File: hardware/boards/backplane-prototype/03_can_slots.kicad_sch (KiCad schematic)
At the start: 17 parts, among them J1 SLOT_1, J2 XY308-2.54-3P / EXTERNAL CAN, J3 SLOT_2, J4 SLOT_3, J6 SLOT_4, J7 SLOT_5, J8 SLOT_6, U5 TCAN3413DR

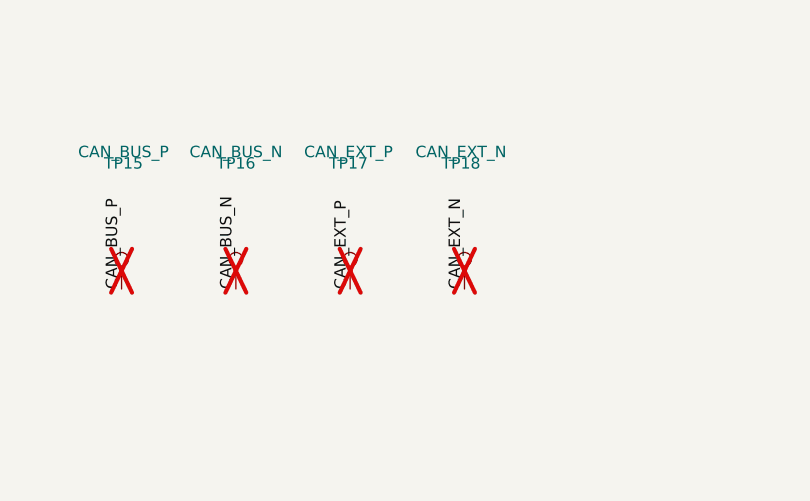
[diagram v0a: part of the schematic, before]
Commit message: checkpoint: save backplane layout updates
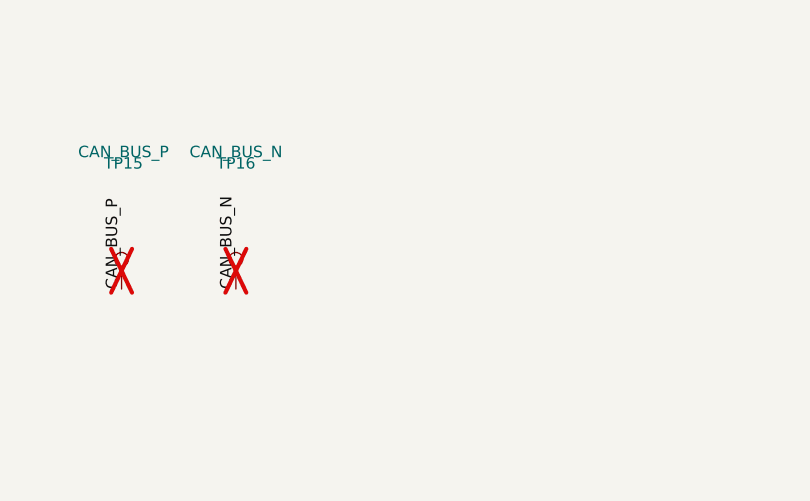
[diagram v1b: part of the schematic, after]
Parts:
- removed TP17: CAN_EXT_P, TestPoint:TestPoint_Pad_D1.5mm, symbol Connector:TestPoint
- removed TP18: CAN_EXT_N, TestPoint:TestPoint_Pad_D1.5mm, symbol Connector:TestPoint
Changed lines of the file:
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@@
-		)
-	)
-	(label "CAN_EXT_N"
-		(at 262.89 44.45 90)
-		(effects
-			(font
-				(size 1.27 1.27)
-			)
-			(justify left bottom)
 		)
 	)
@@
 	(label "CAN_BUS_P"
 		(at 39.37 132.08 0)
-		(effects
-			(font
-				(size 1.27 1.27)
-			)
-			(justify left bottom)
-		)
-	)
-	(label "CAN_EXT_P"
-		(at 250.19 44.45 90)
 		(effects
 			(font
@@
 	)
 	(symbol
-		(lib_id "Connector:TestPoint")
-		(at 262.89 44.45 0)
-		(unit 1)
-		(body_style 1)
-		(exclude_from_sim no)
-		(in_bom no)
-		(on_board yes)
-		(in_pos_files yes)
-		(dnp yes)
-		(property "Reference" "TP18"
-			(at 262.5 30.48 0)
-			(show_name no)
-			(do_not_autoplace no)
-			(effects
-				(font
-					(size 1.27 1.27)
-				)
-			)
-		)
-		(property "Value" "CAN_EXT_N"
-			(at 262.5 29.21 0)
-			(show_name no)
-			(do_not_autoplace no)
-			(effects
-				(font
-					(size 1.27 1.27)
-				)
-			)
-		)
-		(property "Footprint" "TestPoint:TestPoint_Pad_D1.5mm"
-			(at 267.58 45 0)
-			(hide yes)
-			(show_name no)
-			(do_not_autoplace no)
-			(effects
-				(font
-					(size 1.27 1.27)
-				)
-			)
-		)
-		(property "Datasheet" ""
-			(at 267.58 45 0)
-			(hide yes)
-			(show_name no)
-			(do_not_autoplace no)
-			(effects
-				(font
-					(size 1.27 1.27)
-				)
-			)
-		)
-		(property "Description" "test point"
-			(at 262.5 45 0)
-			(hide yes)
-			(show_name no)
-			(do_not_autoplace no)
-			(effects
-				(font
-					(size 1.27 1.27)
-				)
-			)
-		)
-		(pin "1"
-		)
-		(instances
-			(project "backplane-prototype"
-				(path "/348cc909-6345-4013-9bef-98714057a65b/eb7e4e77-e42b-4b43-976a-f7a3e8147b95"
-					(reference "TP18")
-					(unit 1)
-				)
-			)
-		)
-	)
-	(symbol
 		(lib_id "backplane-backpack:ACT1210D_1243")
 		(at 115.57 54.61 0)
@@
 					(unit 1)
 				)
-			)
-		)
-	)
-	(symbol
-		(lib_id "Connector:TestPoint")
-		(at 250.19 44.45 0)
-		(unit 1)
-		(body_style 1)
-		(exclude_from_sim no)
-		(in_bom no)
-		(on_board yes)
-		(in_pos_files yes)
-		(dnp yes)
-		(property "Reference" "TP17"
-			(at 250 30.48 0)
-			(show_name no)
-			(do_not_autoplace no)
-			(effects
-				(font
-					(size 1.27 1.27)
-				)
-			)
-		)
-		(property "Value" "CAN_EXT_P"
-			(at 250 29.21 0)
-			(show_name no)
-			(do_not_autoplace no)
-			(effects
-				(font
-					(size 1.27 1.27)
-				)
-			)
-		)
-		(property "Footprint" "TestPoint:TestPoint_Pad_D1.5mm"
-			(at 255.08 45 0)
-			(hide yes)
-			(show_name no)
-			(do_not_autoplace no)
-			(effects
-				(font
-					(size 1.27 1.27)
-				)
-			)
-		)
-		(property "Datasheet" ""
-			(at 255.08 45 0)
-			(hide yes)
-			(show_name no)
-			(do_not_autoplace no)
-			(effects
-				(font
-					(size 1.27 1.27)
-				)
-			)
-		)
-		(property "Description" "test point"
-			(at 250 45 0)
-			(hide yes)
-			(show_name no)
-			(do_not_autoplace no)
-			(effects
-				(font
-					(size 1.27 1.27)
-				)
-			)
-		)
-		(pin "1"
-		)
-		(instances
-			(project "backplane-prototype"
-				(path "/348cc909-6345-4013-9bef-98714057a65b/eb7e4e77-e42b-4b43-976a-f7a3e8147b95"
-					(reference "TP17")
-					(unit 1)
-				)
